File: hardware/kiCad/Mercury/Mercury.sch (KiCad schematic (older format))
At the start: 72 parts, among them J1 SWD, J10 OUTPUT, J11 Analog I/O, J12 Power Rails, J2 UART1, J3 I2C2, J4 UART1, J5 SPI1, J6 SPI2, J7 1981568-1, J8 Battery Input, J9 INPUT, Q1 AO3401A, SW1 SW_SPDT, U1 STM32F407VGT6, U2 AMS1117-3.3, U3 AMS1117-5.0, Y1 HSE 16MHz

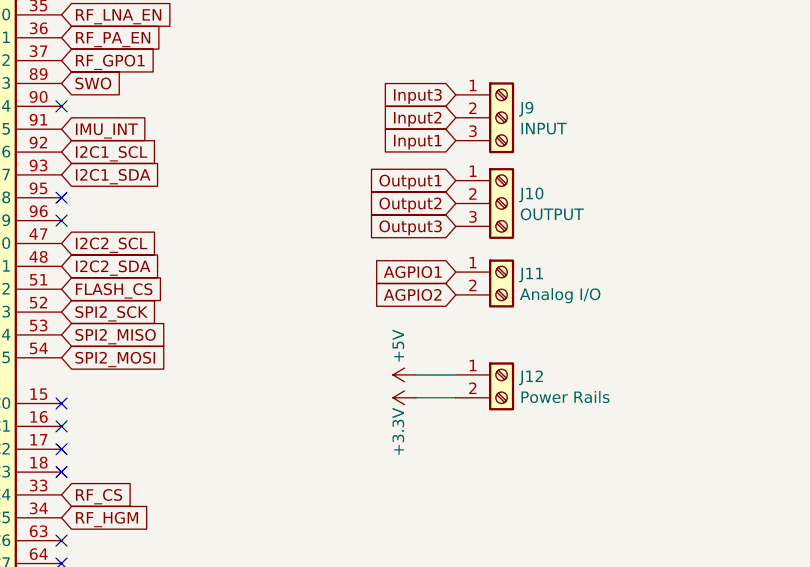
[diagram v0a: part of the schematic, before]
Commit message: Layout + Routing v1 done
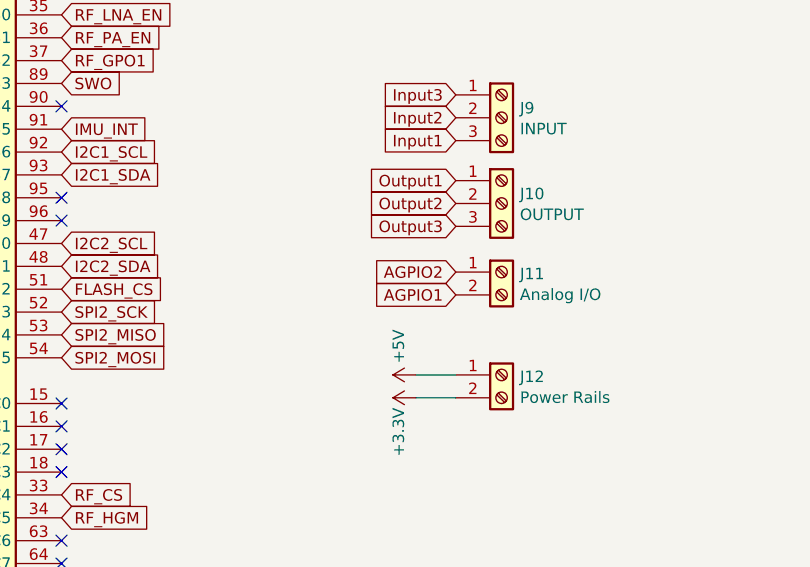
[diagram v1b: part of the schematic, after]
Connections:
- net AGPIO1: now also J11.2 (Pin_2); no longer J11.1 (Pin_1)
- net AGPIO2: now also J11.1 (Pin_1); no longer J11.2 (Pin_2)
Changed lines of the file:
@@
 	1    0    0    -1
 $EndComp
+Text GLabel 6025 4725 0    50   Input ~ 0
+AGPIO1
 Text GLabel 6025 4625 0    50   Input ~ 0
-AGPIO1
-Text GLabel 6025 4725 0    50   Input ~ 0
 AGPIO2
 Text GLabel 6025 4225 0    50   Input ~ 0
